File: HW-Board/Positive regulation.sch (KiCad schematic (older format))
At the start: 16 parts, among them Q2 Si4435, U2 MCP4725, U3 AD5245, U4 OP07, U5 INA219POS

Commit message: sync
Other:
- note added: "LM395 ?"
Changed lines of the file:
@@
 	1    0    0    -1
 $EndComp
+Text Notes 6350 2200 0    50   ~ 0
+LM395  ?
 $EndSCHEMATC

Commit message: SYNC
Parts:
- Q2: symbol Peters:Si4435 -> BreadbaordPSU-rescue:Si4435-Peters
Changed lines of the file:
@@
 VposOut
 $Comp
-L Peters:Si4435 Q?
+L BreadbaordPSU-rescue:Si4435-Peters Q?
 U 1 1 5CFA01F0
 P 6400 2650
 AR Path="/5CFAD453/5CFA01F0" Ref="Q?"  Part="1"
 AR Path="/5CF8F081/5CFA01F0" Ref="Q2"  Part="1"
+AR Path="/5CFA01F0" Ref="Q2"  Part="1"
 F 0 "Q2" V 6743 2650 50  0000 C CNN
 F 1 "Si4435" V 6652 2650 50  0000 C CNN

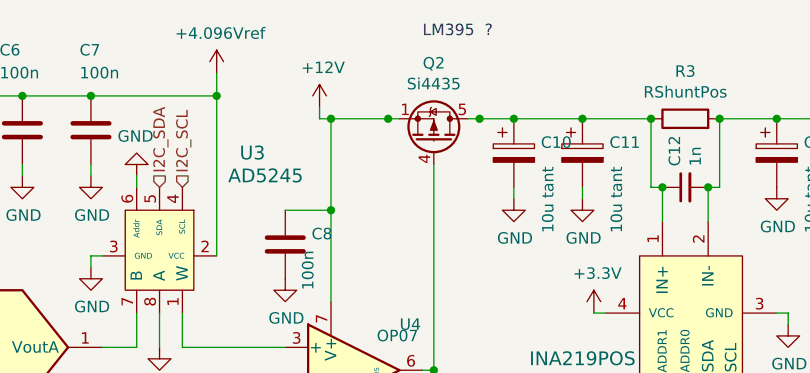
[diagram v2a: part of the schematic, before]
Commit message: sync
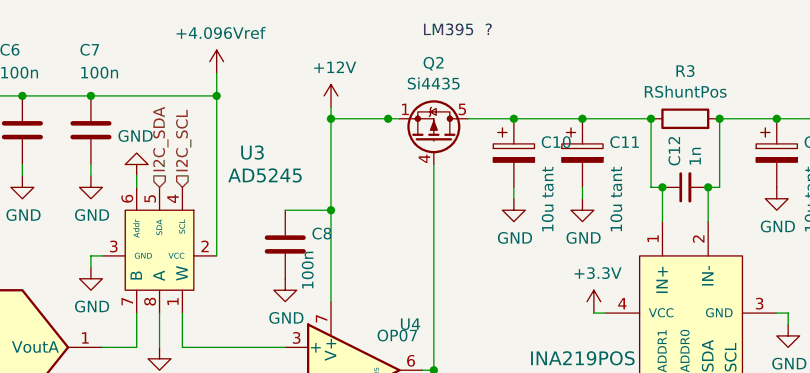
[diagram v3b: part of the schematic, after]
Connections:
- net at C10.1, C11.1, C12.1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: no longer Q2.6 (D), Q2.7 (D), Q2.8 (D)
- new net: Q2.6 (D), Q2.7 (D), Q2.8 (D)
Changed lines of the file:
@@
 	1    0    0    -1
 $EndComp
-Wire Wire Line
-	6750 2550 6600 2550
 Connection ~ 6750 2550
-Connection ~ 6600 2550
-Wire Wire Line
-	6600 2550 6550 2550
 $Comp
 L power:+12V #PWR?
 U 1 1 5CFA0200
-P 5900 2500
+P 5950 2500
 AR Path="/5CFA0200" Ref="#PWR?"  Part="1"
 AR Path="/5CFAD453/5CFA0200" Ref="#PWR?"  Part="1"
 AR Path="/5CF8F081/5CFA0200" Ref="#PWR0127"  Part="1"
-F 0 "#PWR0127" H 5900 2350 50  0001 C CNN
-F 1 "+12V" H 5915 2673 50  0000 C CNN
-F 2 "" H 5900 2500 50  0001 C CNN
-F 3 "" H 5900 2500 50  0001 C CNN
-	1    5900 2500
+F 0 "#PWR0127" H 5950 2350 50  0001 C CNN
+F 1 "+12V" H 5965 2673 50  0000 C CNN
+F 2 "" H 5950 2500 50  0001 C CNN
+F 3 "" H 5950 2500 50  0001 C CNN
+	1    5950 2500
 	1    0    0    -1
 $EndComp
@@
 	6250 2550 6200 2550
 Wire Wire Line
-	5900 2550 5900 2500
+	5950 2550 5950 2500
 Connection ~ 6200 2550
 Wire Wire Line
@@
 I2C_SCL
 Connection ~ 5950 2550
-Wire Wire Line
-	5950 2550 5900 2550
 $Comp
 L Device:C C?
@@
 Text Notes 6350 2200 0    50   ~ 0
 LM395  ?
+Wire Wire Line
+	6550 2550 6750 2550
 $EndSCHEMATC
